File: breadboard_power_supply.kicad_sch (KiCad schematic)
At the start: 17 parts, among them J1 Conn_01x02_Pin, J2 Conn_01x02_Pin, J3 Conn_01x03_Pin, J4 Conn_01x03_Pin, J5 Screw_Terminal_01x02, J6 Barrel_Jack_Switch, J7 Screw_Terminal_01x02, U2 LM317_TO-220, U3 LM7805_TO220

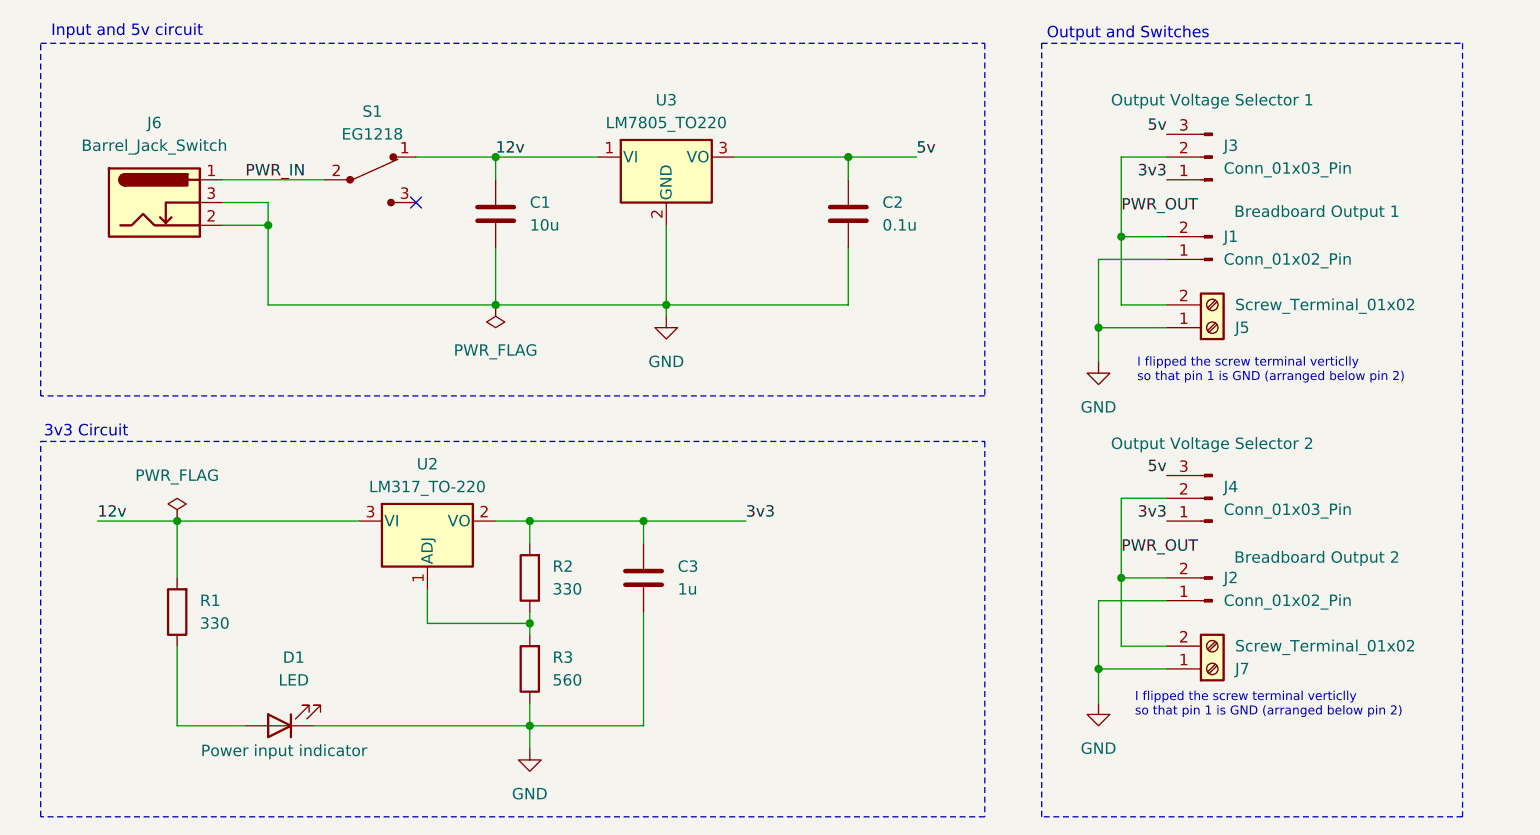
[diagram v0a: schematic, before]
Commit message: v0.1
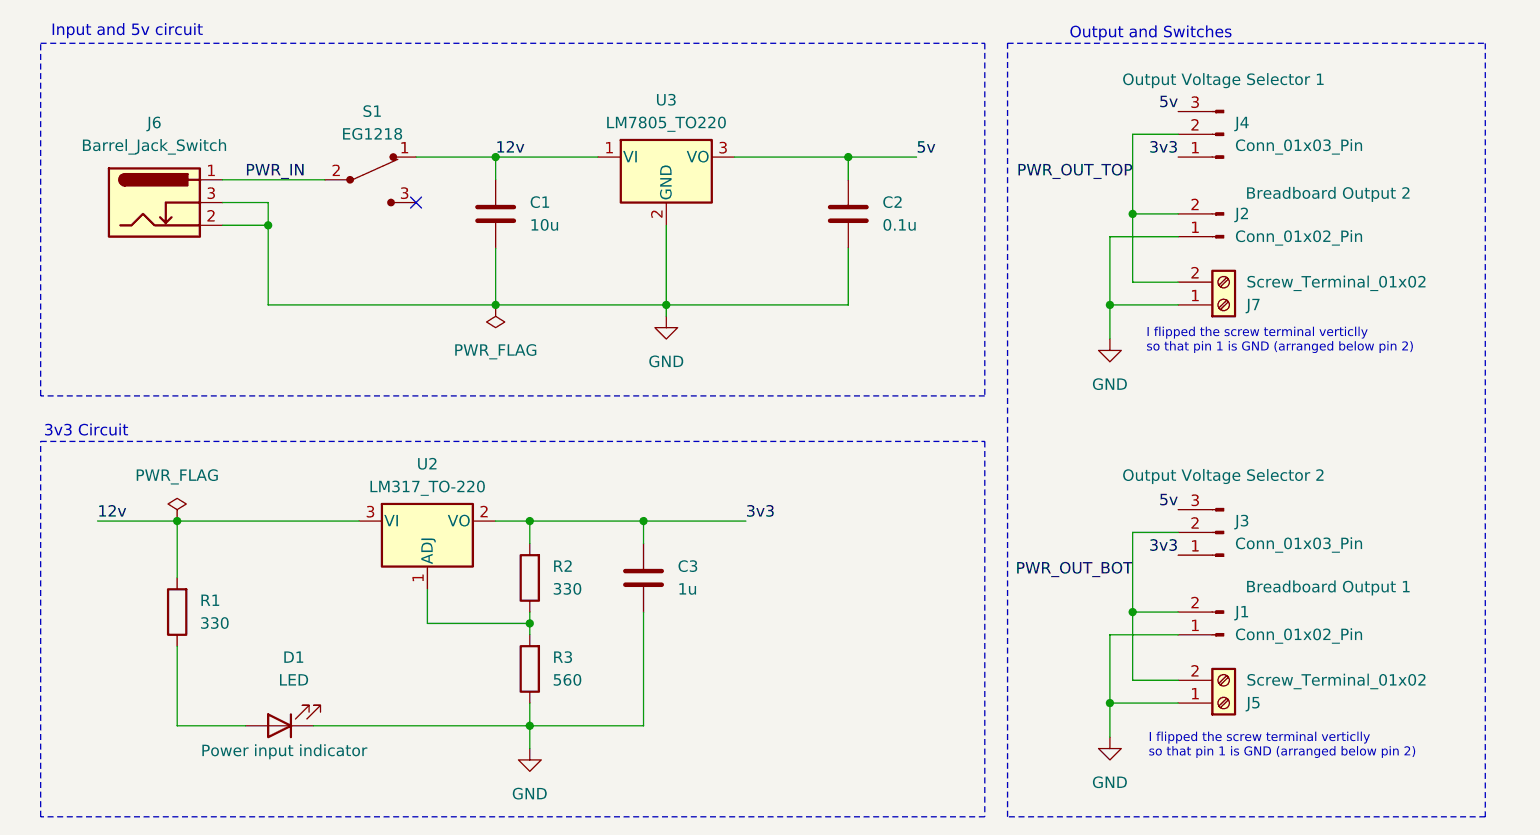
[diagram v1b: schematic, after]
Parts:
- J3: Purpose Output Voltage Selector 1 -> Output Voltage Selector 2
- J4: Purpose Output Voltage Selector 2 -> Output Voltage Selector 1
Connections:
- net PWR_OUT renamed PWR_OUT_BOT
- net PWR_OUT_BOT: no longer J2.2 (Pin_2), J4.2 (Pin_2), J7.2 (Pin_2)
- new net PWR_OUT_TOP: J2.2 (Pin_2), J4.2 (Pin_2), J7.2 (Pin_2)
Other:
- moved on the sheet: J1, J2, J3, J4, J5, J7
